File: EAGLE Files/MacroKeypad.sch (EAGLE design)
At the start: 8 parts

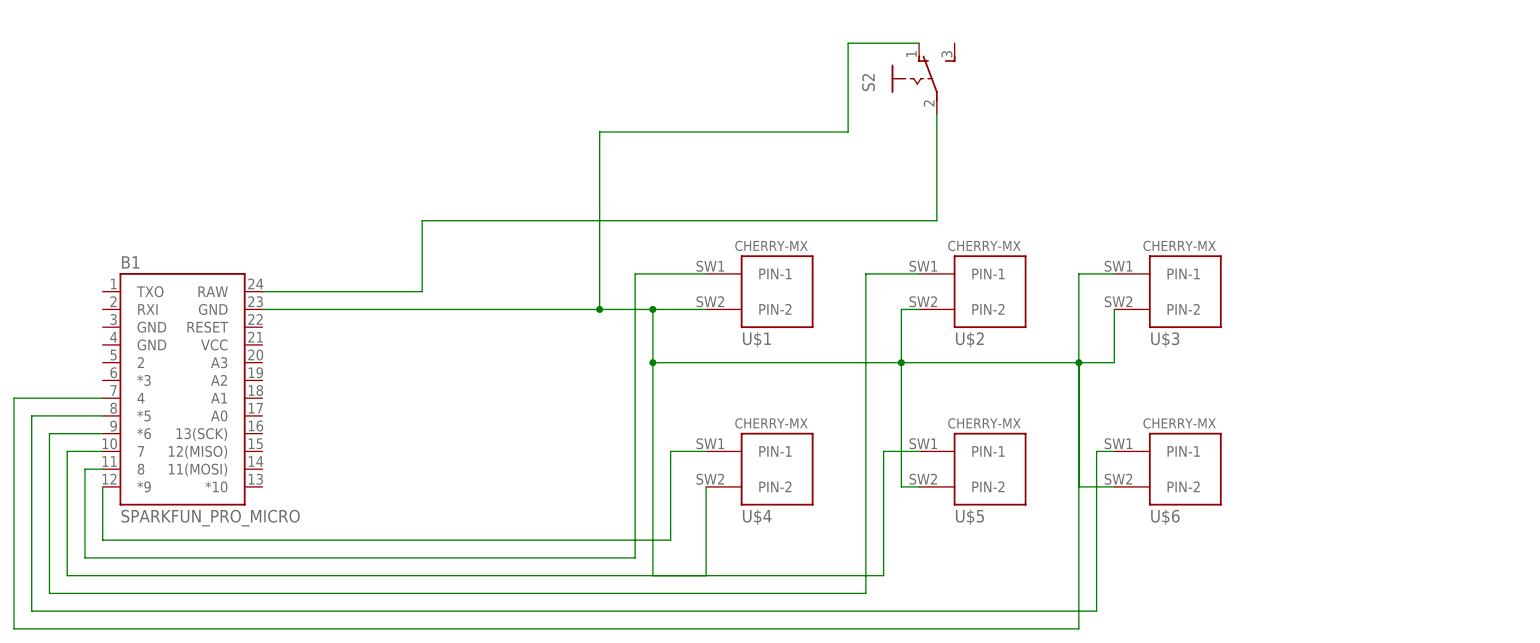
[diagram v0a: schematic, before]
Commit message: Clean up old files
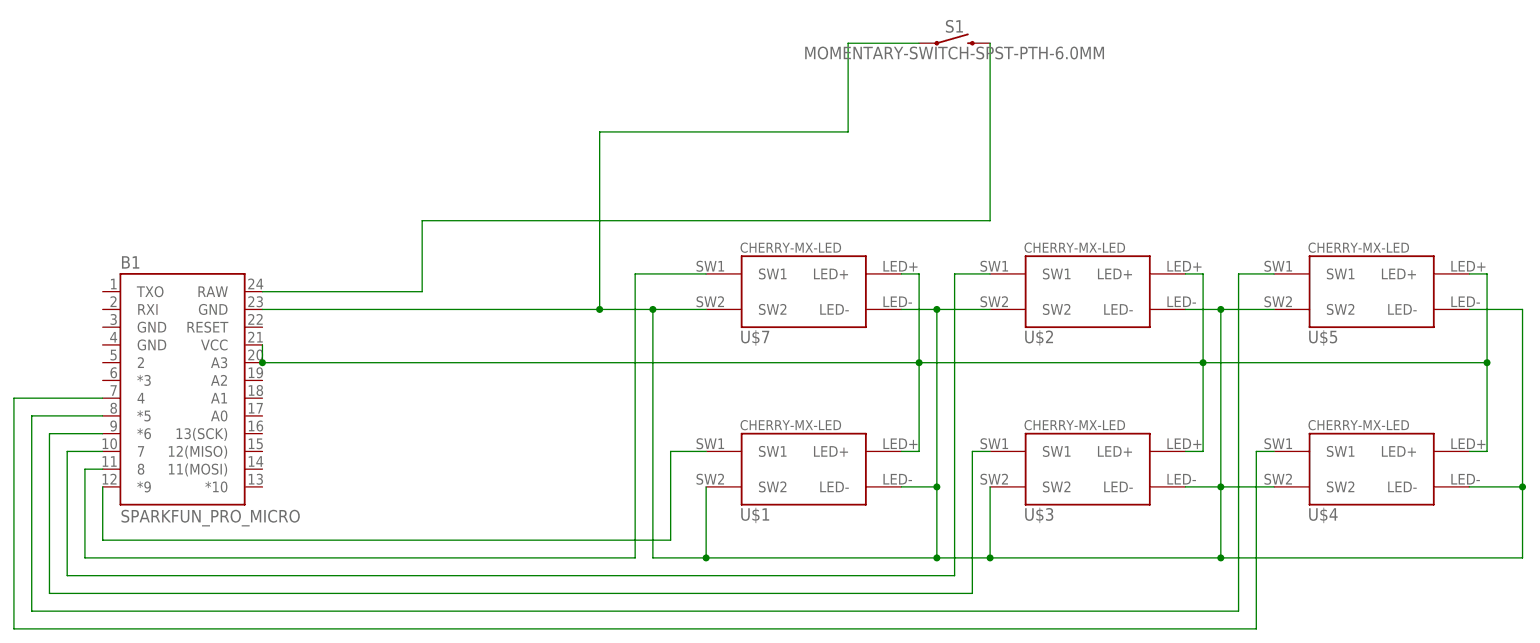
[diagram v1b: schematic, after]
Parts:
- removed S2: (no value), switch:255SB
- removed U$6: CHERRY-MX, cherrymx:CHERRY-MX
- added S1: MOMENTARY-SWITCH-SPST-PTH-6.0MM, SparkFun-Switches:MOMENTARY-SWITCH-SPST-PTH-6.0MM
- added U$7: CHERRY-MX-LED, cherrymx:CHERRY-MX-LED
- U$1, U$2, U$3, U$4, U$5: value CHERRY-MX -> CHERRY-MX-LED; device cherrymx:CHERRY-MX -> cherrymx:CHERRY-MX-LED
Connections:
- new net LED+: B1.A3, B1.VCC, U$1.LED+, U$2.LED+, U$3.LED+, U$4.LED+, U$5.LED+, U$7.LED+
- net GND: now also S1.1, U$1.LED-, U$1.SW2, U$2.LED-, U$2.SW2, U$3.LED-, U$3.SW2, U$4.LED-, U$4.SW2, U$5.LED-, U$5.SW2, U$7.LED-, U$7.SW2; no longer S2.O, U$1.PIN-2, U$2.PIN-2, U$3.PIN-2, U$4.PIN-2, U$5.PIN-2, U$6.PIN-2
- net RESET: now also S1.2; no longer S2.P
- net SW1: now also U$7.SW1; no longer U$1.PIN-1
- net SW2: now also U$3.SW1; no longer U$2.PIN-1
- net SW3: now also U$4.SW1; no longer U$3.PIN-1
- net SW4: now also U$1.SW1; no longer U$4.PIN-1
- net SW5: now also U$2.SW1; no longer U$5.PIN-1
- net SW6: now also U$5.SW1; no longer U$6.PIN-1
